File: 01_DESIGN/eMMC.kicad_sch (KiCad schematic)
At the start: 20 parts, among them U4 MTFC32GAZAQDW-AAT

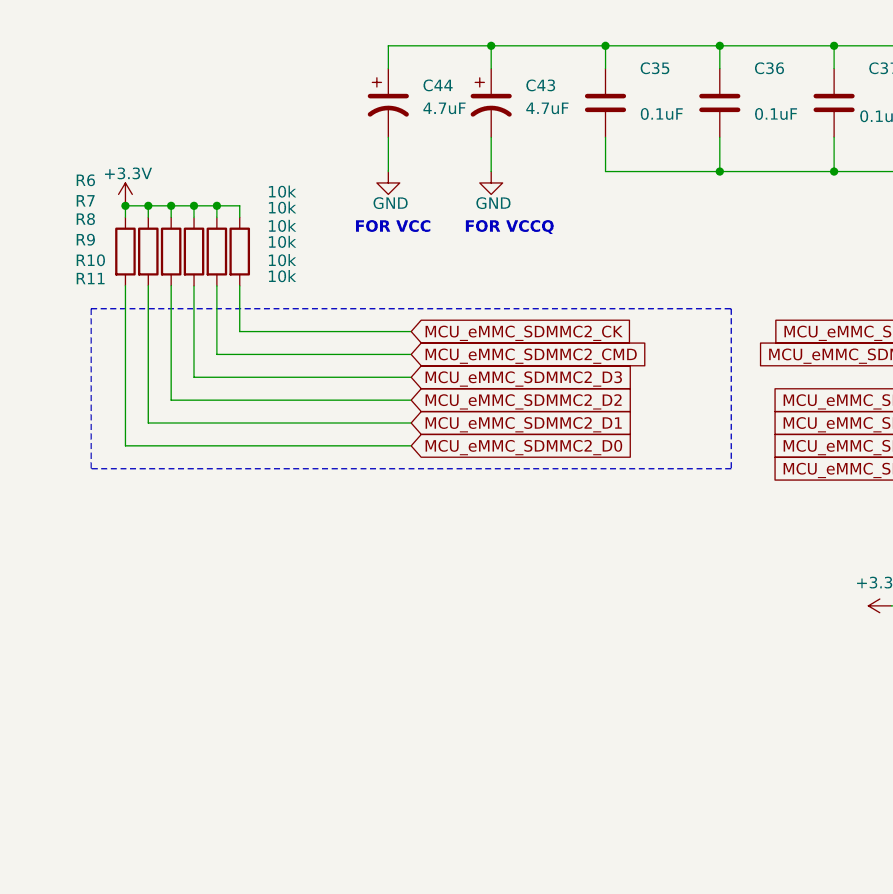
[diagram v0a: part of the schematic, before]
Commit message: Update project
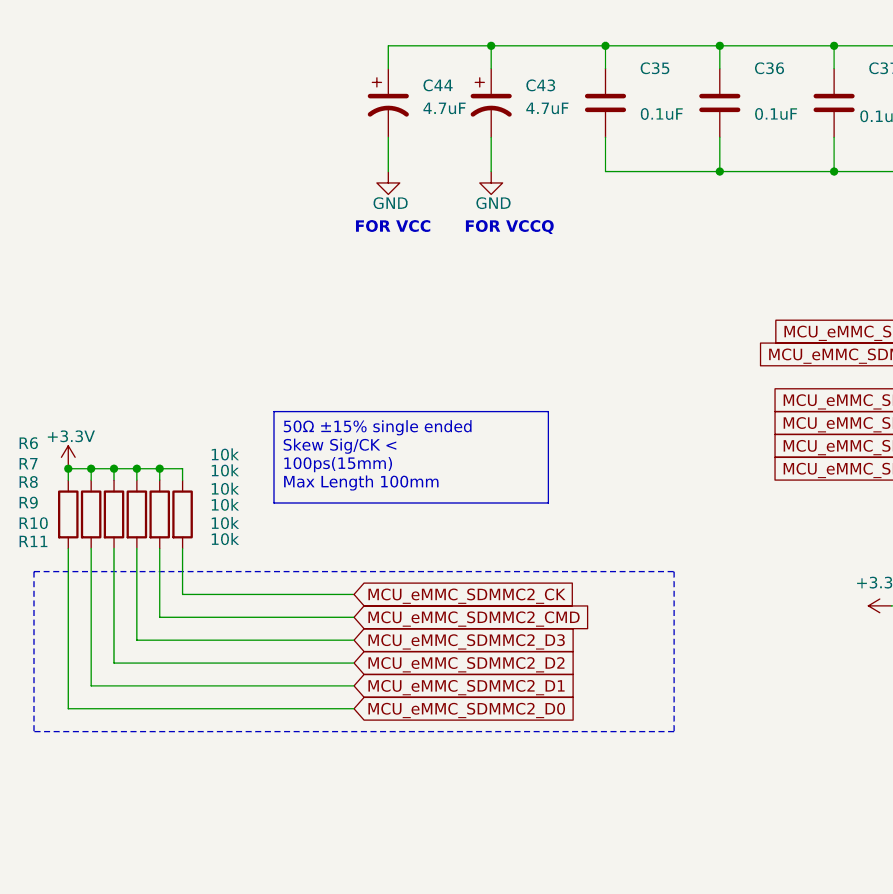
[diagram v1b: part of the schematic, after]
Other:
- moved on the sheet: R10, R11, R6, R7, R8, R9

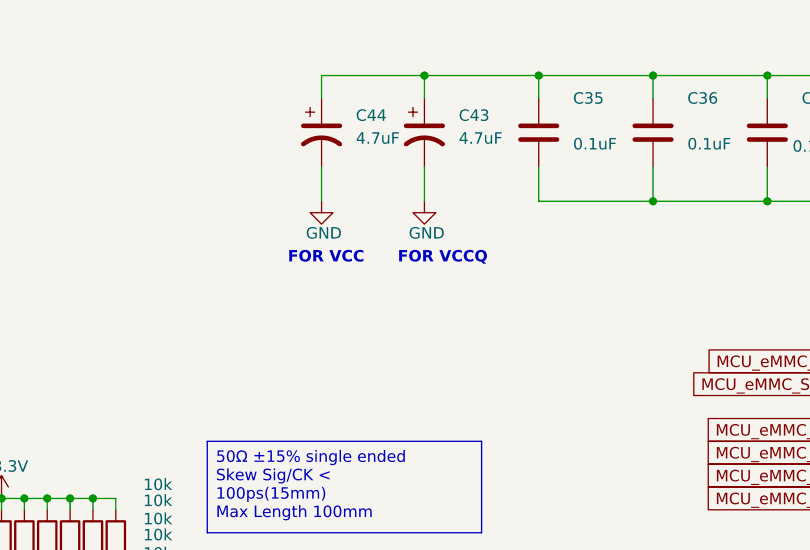
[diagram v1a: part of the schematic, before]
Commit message: Update KiCad project files
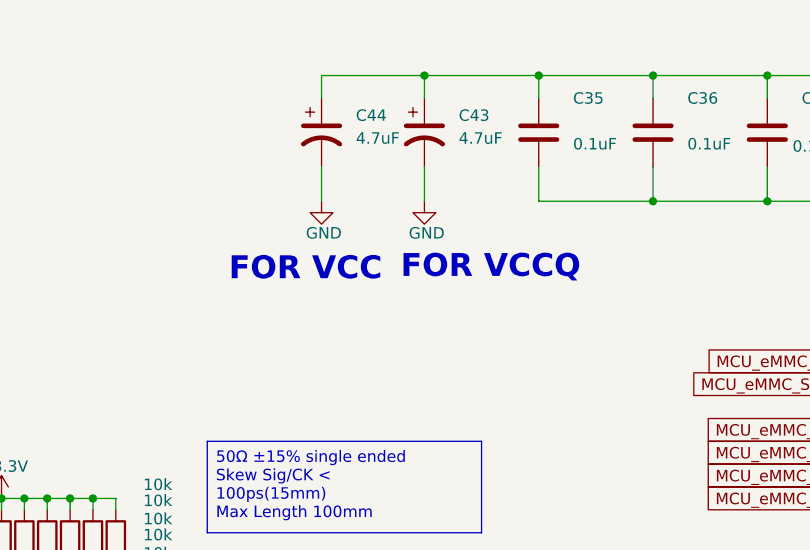
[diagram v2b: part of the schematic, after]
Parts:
- C35, C36, C37, C38, C39, C40, C41, C42, C45: symbol Device:C -> LABLIB:C
- C43, C44, C46: symbol Device:C_Polarized_US -> LABLIB:C_Polarized_US
- R10, R11, R12, R6, R7, R8, R9: symbol Device:R -> LABLIB:R
- U4: symbol AUSB:MTFC32GAZAQDW-AAT -> LABLIB:MTFC32GAZAQDW-AAT
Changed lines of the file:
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@@
 	(generator_version "10.0")
 	(paper "A3")
-	(text "FOR VCCQ\n"
+	(text "FOR VCC"
 		(exclude_from_sim no)
-		(at 76.962 41.91 0)
+		(at 61.722 43.18 0)
 		(effects
 			(font
-				(size 1.27 1.27)
-				(thickness 0.254)
+				(face "Times New Roman")
+				(size 2.54 2.54)
+				(thickness 0.3175)
 				(bold yes)
 			)
 		)
 	)
-	(text "FOR VCC\n"
+	(text "FOR VCCQ"
 		(exclude_from_sim no)
-		(at 64.008 41.91 0)
+		(at 82.296 42.926 0)
 		(effects
 			(font
-				(size 1.27 1.27)
-				(thickness 0.254)
+				(face "Times New Roman")
+				(size 2.54 2.54)
+				(thickness 0.3175)
 				(bold yes)
 			)
@@
 	)
 	(symbol
-		(lib_id "Device:R")
+		(lib_id "LABLIB:R")
 		(at 33.02 73.66 0)
 		(unit 1)
@@
 		)
 		(instances
-			(project "kicad_demo_project"
+			(project "PROJECT_VD_KICAD"
 				(path "/fd6ef0b1-201f-4377-afd7-d57558236c20/bd4f8c4f-5d4d-4af0-bc9a-09e0d8b47729"
 					(reference "R8")
@@
 		)
 		(instances
-			(project "kicad_demo_project"
+			(project "PROJECT_VD_KICAD"
 				(path "/fd6ef0b1-201f-4377-afd7-d57558236c20/bd4f8c4f-5d4d-4af0-bc9a-09e0d8b47729"
 					(reference "#PWR049")
@@
 	)
 	(symbol
-		(lib_id "AUSB:MTFC32GAZAQDW-AAT")
+		(lib_id "LABLIB:MTFC32GAZAQDW-AAT")
 		(at 262.89 76.2 0)
 		(unit 3)
@@
 		)
 		(instances
-			(project "kicad_demo_project"
+			(project "PROJECT_VD_KICAD"
 				(path "/fd6ef0b1-201f-4377-afd7-d57558236c20/bd4f8c4f-5d4d-4af0-bc9a-09e0d8b47729"
 					(reference "U4")
@@
 		)
 		(instances
-			(project "kicad_demo_project"
+			(project "PROJECT_VD_KICAD"
 				(path "/fd6ef0b1-201f-4377-afd7-d57558236c20/bd4f8c4f-5d4d-4af0-bc9a-09e0d8b47729"
 					(reference "#PWR045")
@@
 	)
 	(symbol
-		(lib_id "Device:C_Polarized_US")
+		(lib_id "LABLIB:C_Polarized_US")
 		(at 74.93 27.94 0)
 		(unit 1)
@@
 		)
 		(instances
-			(project "kicad_demo_project"
+			(project "PROJECT_VD_KICAD"
 				(path "/fd6ef0b1-201f-4377-afd7-d57558236c20/bd4f8c4f-5d4d-4af0-bc9a-09e0d8b47729"
 					(reference "C43")
@@
 	)
 	(symbol
-		(lib_id "Device:C")
+		(lib_id "LABLIB:C")
 		(at 234.95 58.42 0)
 		(unit 1)
@@
 		)
 		(instances
-			(project "kicad_demo_project"
+			(project "PROJECT_VD_KICAD"
 				(path "/fd6ef0b1-201f-4377-afd7-d57558236c20/bd4f8c4f-5d4d-4af0-bc9a-09e0d8b47729"
 					(reference "C45")
@@
 	)
 	(symbol
-		(lib_id "Device:C")
+		(lib_id "LABLIB:C")
 		(at 100.33 27.94 0)
 		(unit 1)
@@
 		)
 		(instances
-			(project "kicad_demo_project"
+			(project "PROJECT_VD_KICAD"
 				(path "/fd6ef0b1-201f-4377-afd7-d57558236c20/bd4f8c4f-5d4d-4af0-bc9a-09e0d8b47729"
 					(reference "C36")
@@
 		)
 		(instances
-			(project "kicad_demo_project"
+			(project "PROJECT_VD_KICAD"
 				(path "/fd6ef0b1-201f-4377-afd7-d57558236c20/bd4f8c4f-5d4d-4af0-bc9a-09e0d8b47729"
 					(reference "#PWR053")
@@
 	)
 	(symbol
-		(lib_id "Device:C")
+		(lib_id "LABLIB:C")
 		(at 151.13 27.94 0)
 		(unit 1)
@@
 		)
 		(instances
-			(project "kicad_demo_project"
+			(project "PROJECT_VD_KICAD"
 				(path "/fd6ef0b1-201f-4377-afd7-d57558236c20/bd4f8c4f-5d4d-4af0-bc9a-09e0d8b47729"
 					(reference "C39")
@@
 		)
 		(instances
-			(project "kicad_demo_project"
+			(project "PROJECT_VD_KICAD"
 				(path "/fd6ef0b1-201f-4377-afd7-d57558236c20/bd4f8c4f-5d4d-4af0-bc9a-09e0d8b47729"
 					(reference "#PWR048")
@@
 	)
 	(symbol
-		(lib_id "Device:R")
+		(lib_id "LABLIB:R")
 		(at 27.94 73.66 0)
 		(unit 1)
@@
 		)
 		(instances
-			(project "kicad_demo_project"
+			(project "PROJECT_VD_KICAD"
 				(path "/fd6ef0b1-201f-4377-afd7-d57558236c20/bd4f8c4f-5d4d-4af0-bc9a-09e0d8b47729"
 					(reference "R6")
@@
 		)
 		(instances
-			(project "kicad_demo_project"
+			(project "PROJECT_VD_KICAD"
 				(path "/fd6ef0b1-201f-4377-afd7-d57558236c20/bd4f8c4f-5d4d-4af0-bc9a-09e0d8b47729"
 					(reference "#PWR046")
@@
 	)
 	(symbol
-		(lib_id "Device:R")
+		(lib_id "LABLIB:R")
 		(at 38.1 73.66 0)
 		(unit 1)
@@
 		)
 		(instances
-			(project "kicad_demo_project"
+			(project "PROJECT_VD_KICAD"
 				(path "/fd6ef0b1-201f-4377-afd7-d57558236c20/bd4f8c4f-5d4d-4af0-bc9a-09e0d8b47729"
 					(reference "R10")
@@
 		)
 		(instances
-			(project "kicad_demo_project"
+			(project "PROJECT_VD_KICAD"
 				(path "/fd6ef0b1-201f-4377-afd7-d57558236c20/bd4f8c4f-5d4d-4af0-bc9a-09e0d8b47729"
 					(reference "#PWR044")
@@
 	)
 	(symbol
-		(lib_id "Device:C")
+		(lib_id "LABLIB:C")
 		(at 113.03 27.94 0)
 		(unit 1)
@@
 		)
 		(instances
-			(project "kicad_demo_project"
+			(project "PROJECT_VD_KICAD"
 				(path "/fd6ef0b1-201f-4377-afd7-d57558236c20/bd4f8c4f-5d4d-4af0-bc9a-09e0d8b47729"
 					(reference "C37")
@@
 	)
 	(symbol
-		(lib_id "Device:C_Polarized_US")
+		(lib_id "LABLIB:C_Polarized_US")
 		(at 63.5 27.94 0)
 		(unit 1)
@@
 		)
 		(instances
-			(project "kicad_demo_project"
+			(project "PROJECT_VD_KICAD"
 				(path "/fd6ef0b1-201f-4377-afd7-d57558236c20/bd4f8c4f-5d4d-4af0-bc9a-09e0d8b47729"
 					(reference "C44")
@@
 		)
 		(instances
-			(project "kicad_demo_project"
+			(project "PROJECT_VD_KICAD"
 				(path "/fd6ef0b1-201f-4377-afd7-d57558236c20/bd4f8c4f-5d4d-4af0-bc9a-09e0d8b47729"
 					(reference "#PWR047")
@@
 	)
 	(symbol
-		(lib_id "Device:C")
+		(lib_id "LABLIB:C")
 		(at 189.23 27.94 0)
 		(unit 1)
@@
 		)
 		(instances
-			(project "kicad_demo_project"
+			(project "PROJECT_VD_KICAD"
 				(path "/fd6ef0b1-201f-4377-afd7-d57558236c20/bd4f8c4f-5d4d-4af0-bc9a-09e0d8b47729"
 					(reference "C42")
@@
 		)
 		(instances
-			(project "kicad_demo_project"
+			(project "PROJECT_VD_KICAD"
 				(path "/fd6ef0b1-201f-4377-afd7-d57558236c20/bd4f8c4f-5d4d-4af0-bc9a-09e0d8b47729"
 					(reference "#PWR052")
@@
 	)
 	(symbol
-		(lib_id "Device:C_Polarized_US")
+		(lib_id "LABLIB:C_Polarized_US")
 		(at 223.52 58.42 0)
 		(unit 1)
@@
 		)
 		(instances
-			(project "kicad_demo_project"
+			(project "PROJECT_VD_KICAD"
 				(path "/fd6ef0b1-201f-4377-afd7-d57558236c20/bd4f8c4f-5d4d-4af0-bc9a-09e0d8b47729"
 					(reference "C46")
@@
 	)
 	(symbol
-		(lib_id "AUSB:MTFC32GAZAQDW-AAT")
+		(lib_id "LABLIB:MTFC32GAZAQDW-AAT")
 		(at 194.31 88.9 0)
 		(unit 2)
@@
 		)
 		(instances
-			(project "kicad_demo_project"
+			(project "PROJECT_VD_KICAD"
 				(path "/fd6ef0b1-201f-4377-afd7-d57558236c20/bd4f8c4f-5d4d-4af0-bc9a-09e0d8b47729"
 					(reference "U4")
@@
 	)
 	(symbol
-		(lib_id "AUSB:MTFC32GAZAQDW-AAT")
+		(lib_id "LABLIB:MTFC32GAZAQDW-AAT")
 		(at 148.59 68.58 0)
 		(unit 1)
@@
 		)
 		(instances
-			(project "kicad_demo_project"
+			(project "PROJECT_VD_KICAD"
 				(path "/fd6ef0b1-201f-4377-afd7-d57558236c20/bd4f8c4f-5d4d-4af0-bc9a-09e0d8b47729"
 					(reference "U4")
@@
 	)
 	(symbol
-		(lib_id "Device:R")
+		(lib_id "LABLIB:R")
 		(at 30.48 73.66 0)
 		(unit 1)
@@
 		)
 		(instances
-			(project "kicad_demo_project"
+			(project "PROJECT_VD_KICAD"
 				(path "/fd6ef0b1-201f-4377-afd7-d57558236c20/bd4f8c4f-5d4d-4af0-bc9a-09e0d8b47729"
 					(reference "R7")
@@
 		)
 		(instances
-			(project "kicad_demo_project"
+			(project "PROJECT_VD_KICAD"
 				(path "/fd6ef0b1-201f-4377-afd7-d57558236c20/bd4f8c4f-5d4d-4af0-bc9a-09e0d8b47729"
 					(reference "#PWR050")
@@
 	)
 	(symbol
-		(lib_id "Device:C")
+		(lib_id "LABLIB:C")
 		(at 124.46 27.94 0)
 		(unit 1)
@@
 		)
 		(instances
-			(project "kicad_demo_project"
+			(project "PROJECT_VD_KICAD"
 				(path "/fd6ef0b1-201f-4377-afd7-d57558236c20/bd4f8c4f-5d4d-4af0-bc9a-09e0d8b47729"
 					(reference "C38")
@@
 		)
 		(instances
-			(project "kicad_demo_project"
+			(project "PROJECT_VD_KICAD"
 				(path "/fd6ef0b1-201f-4377-afd7-d57558236c20/bd4f8c4f-5d4d-4af0-bc9a-09e0d8b47729"
 					(reference "#PWR051")
@@
 		)
 		(instances
-			(project "kicad_demo_project"
+			(project "PROJECT_VD_KICAD"
 				(path "/fd6ef0b1-201f-4377-afd7-d57558236c20/bd4f8c4f-5d4d-4af0-bc9a-09e0d8b47729"
 					(reference "#PWR08")
@@
 	)
 	(symbol
-		(lib_id "Device:R")
+		(lib_id "LABLIB:R")
 		(at 40.64 73.66 0)
 		(unit 1)
@@
 		)
 		(instances
-			(project "kicad_demo_project"
+			(project "PROJECT_VD_KICAD"
 				(path "/fd6ef0b1-201f-4377-afd7-d57558236c20/bd4f8c4f-5d4d-4af0-bc9a-09e0d8b47729"
 					(reference "R11")
@@
 	)
 	(symbol
-		(lib_id "Device:C")
+		(lib_id "LABLIB:C")
 		(at 163.83 27.94 0)
 		(unit 1)
@@
 		)
 		(instances
-			(project "kicad_demo_project"
+			(project "PROJECT_VD_KICAD"
 				(path "/fd6ef0b1-201f-4377-afd7-d57558236c20/bd4f8c4f-5d4d-4af0-bc9a-09e0d8b47729"
 					(reference "C40")
@@
 	)
 	(symbol
-		(lib_id "Device:C")
+		(lib_id "LABLIB:C")
 		(at 176.53 27.94 0)
 		(unit 1)
@@
 		)
 		(instances
-			(project "kicad_demo_project"
+			(project "PROJECT_VD_KICAD"
 				(path "/fd6ef0b1-201f-4377-afd7-d57558236c20/bd4f8c4f-5d4d-4af0-bc9a-09e0d8b47729"
 					(reference "C41")
@@
 	)
 	(symbol
-		(lib_id "Device:C")
+		(lib_id "LABLIB:C")
 		(at 87.63 27.94 0)
 		(unit 1)
@@
 		)
 		(instances
-			(project "kicad_demo_project"
+			(project "PROJECT_VD_KICAD"
 				(path "/fd6ef0b1-201f-4377-afd7-d57558236c20/bd4f8c4f-5d4d-4af0-bc9a-09e0d8b47729"
 					(reference "C35")
@@
 	)
 	(symbol
-		(lib_id "Device:R")
+		(lib_id "LABLIB:R")
 		(at 35.56 73.66 0)
 		(unit 1)
@@
 		)
 		(instances
-			(project "kicad_demo_project"
+			(project "PROJECT_VD_KICAD"
 				(path "/fd6ef0b1-201f-4377-afd7-d57558236c20/bd4f8c4f-5d4d-4af0-bc9a-09e0d8b47729"
 					(reference "R9")
@@
 	)
 	(symbol
-		(lib_id "Device:R")
+		(lib_id "LABLIB:R")
 		(at 128.27 83.82 270)
 		(unit 1)
@@
 		)
 		(instances
-			(project "kicad_demo_project"
+			(project "PROJECT_VD_KICAD"
 				(path "/fd6ef0b1-201f-4377-afd7-d57558236c20/bd4f8c4f-5d4d-4af0-bc9a-09e0d8b47729"
 					(reference "R12")
